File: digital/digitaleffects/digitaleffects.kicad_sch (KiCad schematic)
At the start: 20 parts

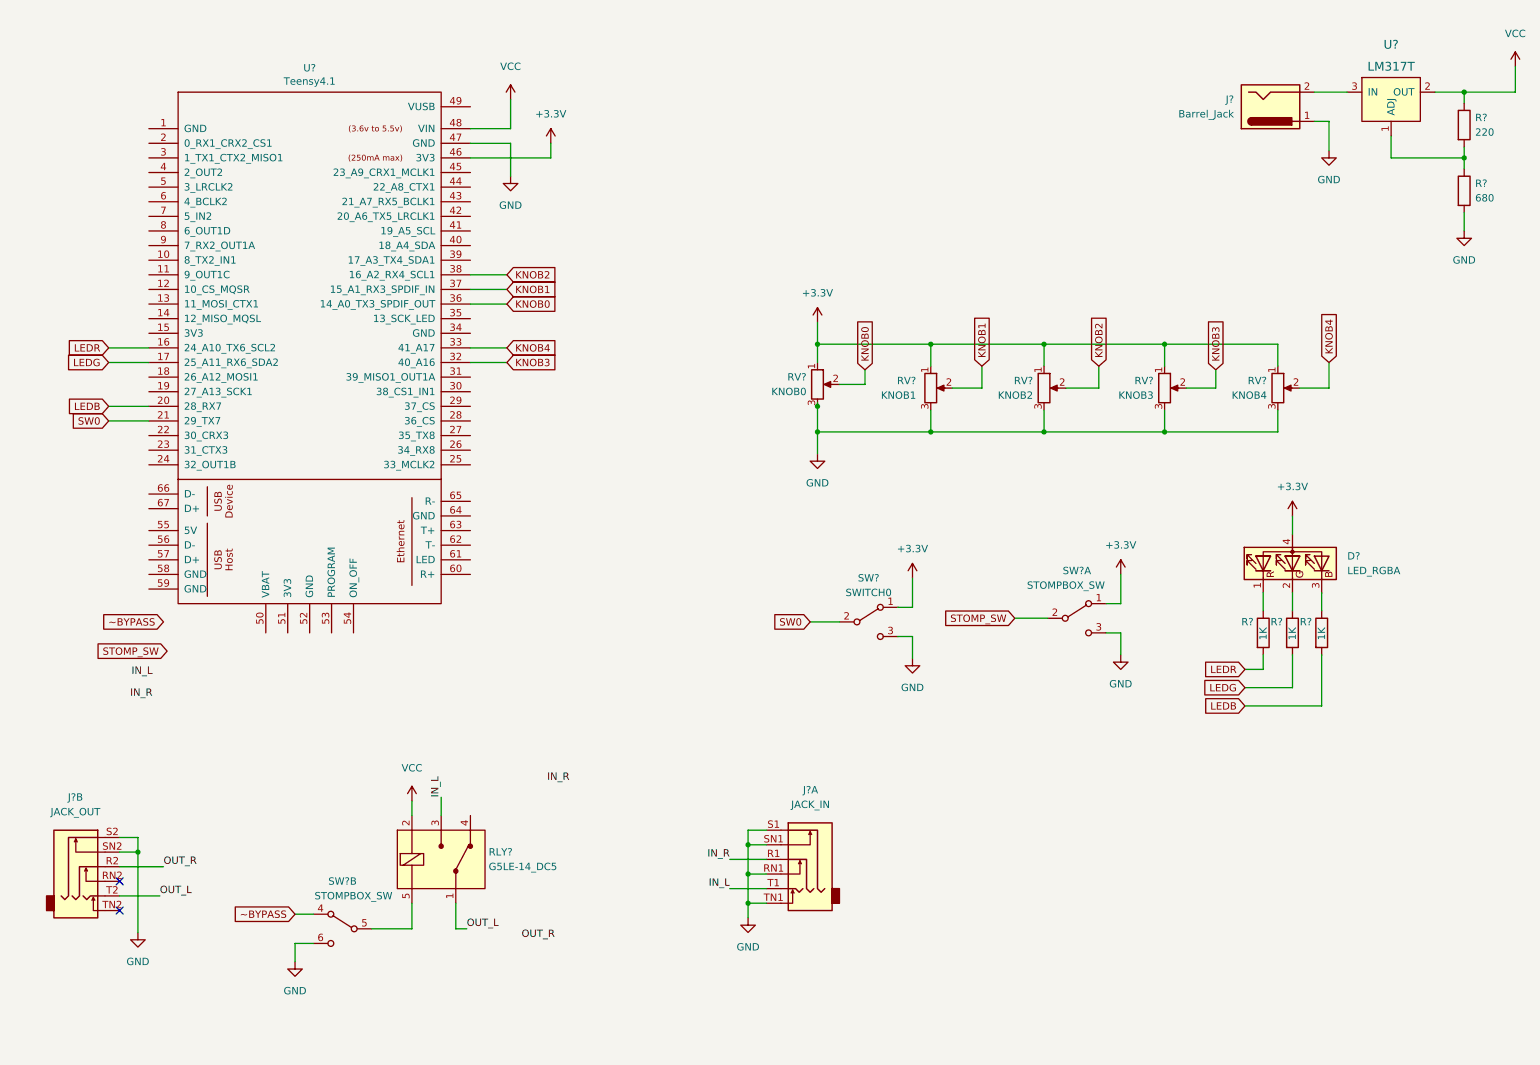
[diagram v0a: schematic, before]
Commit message: proved out all the components
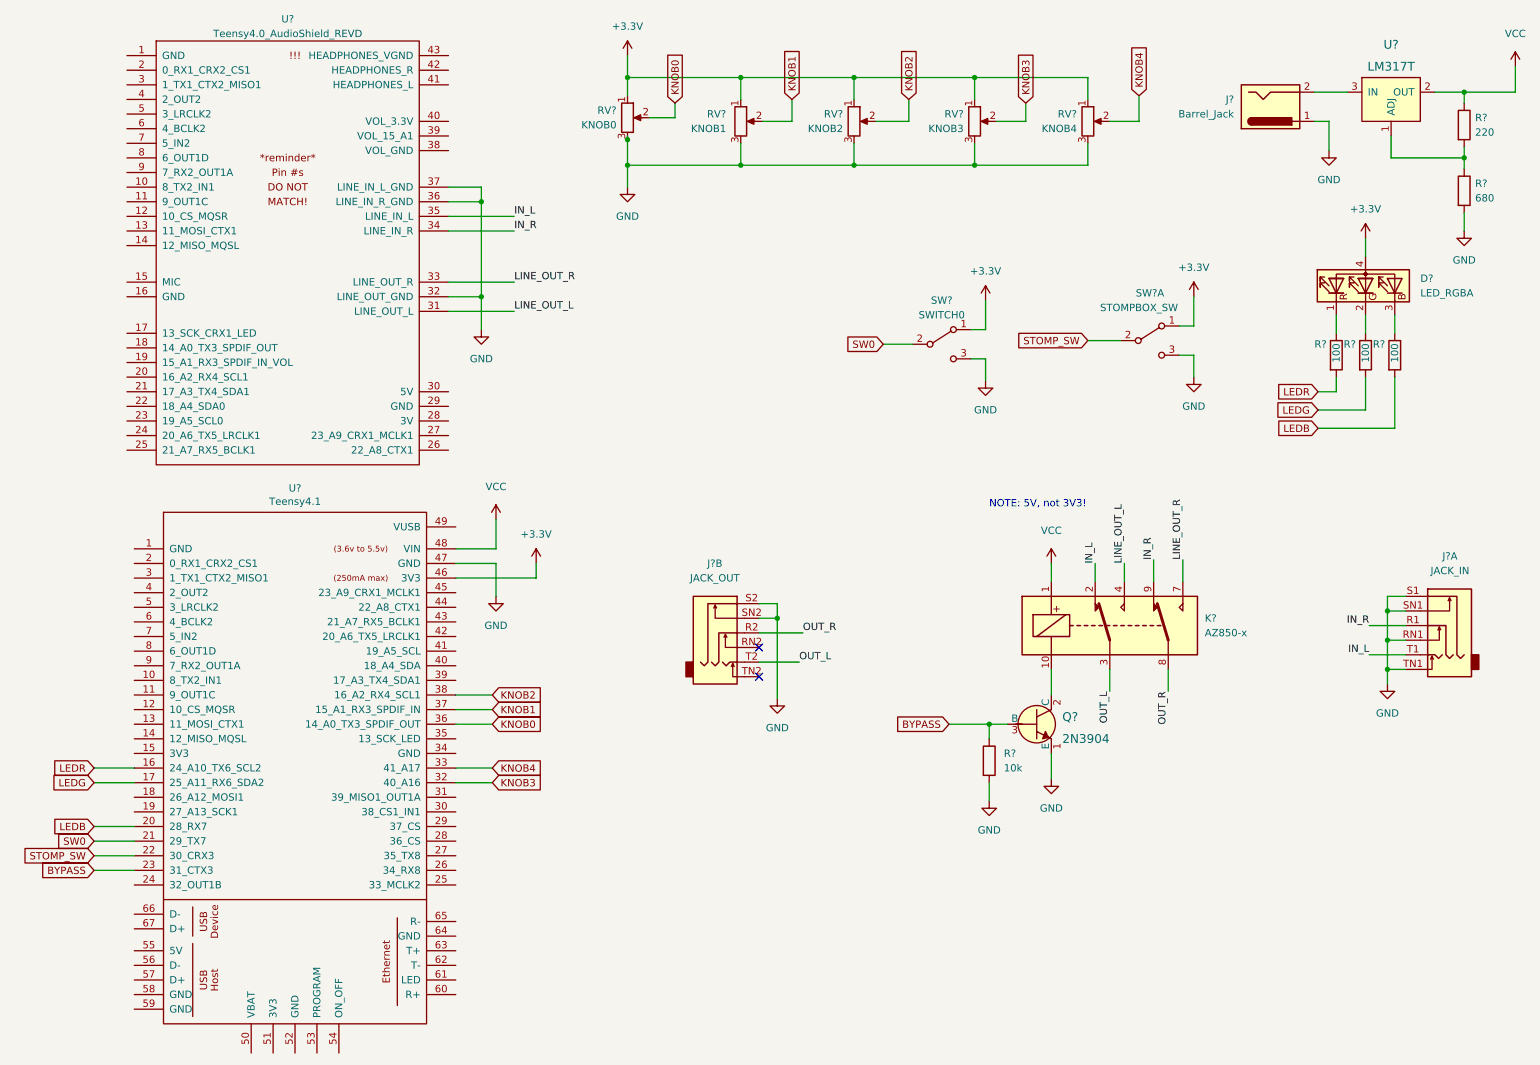
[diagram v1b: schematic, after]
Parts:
- removed RLY?: G5LE-14_DC5, digikey-footprints:Relay_THT_G5LE-14, symbol dk_Power-Relays-Over-2-Amps:G5LE-14_DC5
- removed SW?: STOMPBOX_SW, symbol _effects_shared:SW_3PDT_x3-Switch
- added K?: AZ850-x, Relay_THT:Relay_DPDT_FRT5, symbol Relay:AZ850-x
- added Q?: 2N3904, digikey-footprints:TO-92-3, symbol dk_Transistors-Bipolar-BJT-Single:2N3904
- added R?: 10k, symbol Device:R
- added U?: Teensy4.0_AudioShield_REVD, symbol _proj:Teensy4.0_AudioShield_REVD
- R? (x3): value 1K -> 100
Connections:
- net GND: now also Q?.1 (E), R?.2, U?.32 (LINE_OUT_GND), U?.36 (LINE_IN_R_GND), U?.37 (LINE_IN_L_GND)
- net IN_L: now also K?.2, U?.35 (LINE_IN_L)
- net IN_R: now also K?.9, U?.34 (LINE_IN_R)
- net OUT_L: now also K?.3
- net OUT_R: now also K?.8
- net STOMP_SW: now also U?.22 (30_CRX3)
- net VCC: now also K?.1
- net BYPASS: now reaches U?.23 (31_CTX3)
- net BYPASS: now also Q?.3 (B), R?.1
- new net: K?.10, Q?.2 (C)
- new net LINE_OUT_L: K?.4, U?.31 (LINE_OUT_L)
- new net LINE_OUT_R: K?.7, U?.33 (LINE_OUT_R)
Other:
- note added: "NOTE: 5V, not 3V3!"
- moved on the sheet: D?, J?A, J?B, R?, RV?, SW?, SW?A, U?
